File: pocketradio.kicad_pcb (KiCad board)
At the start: 2 copper layers, 30 x 30 mm, 23 parts, among them CN1 PJ-320D, U1 SI4702-C19-GMR, U2 CH32V003F4U6, U3 TPA6130A2RTJR

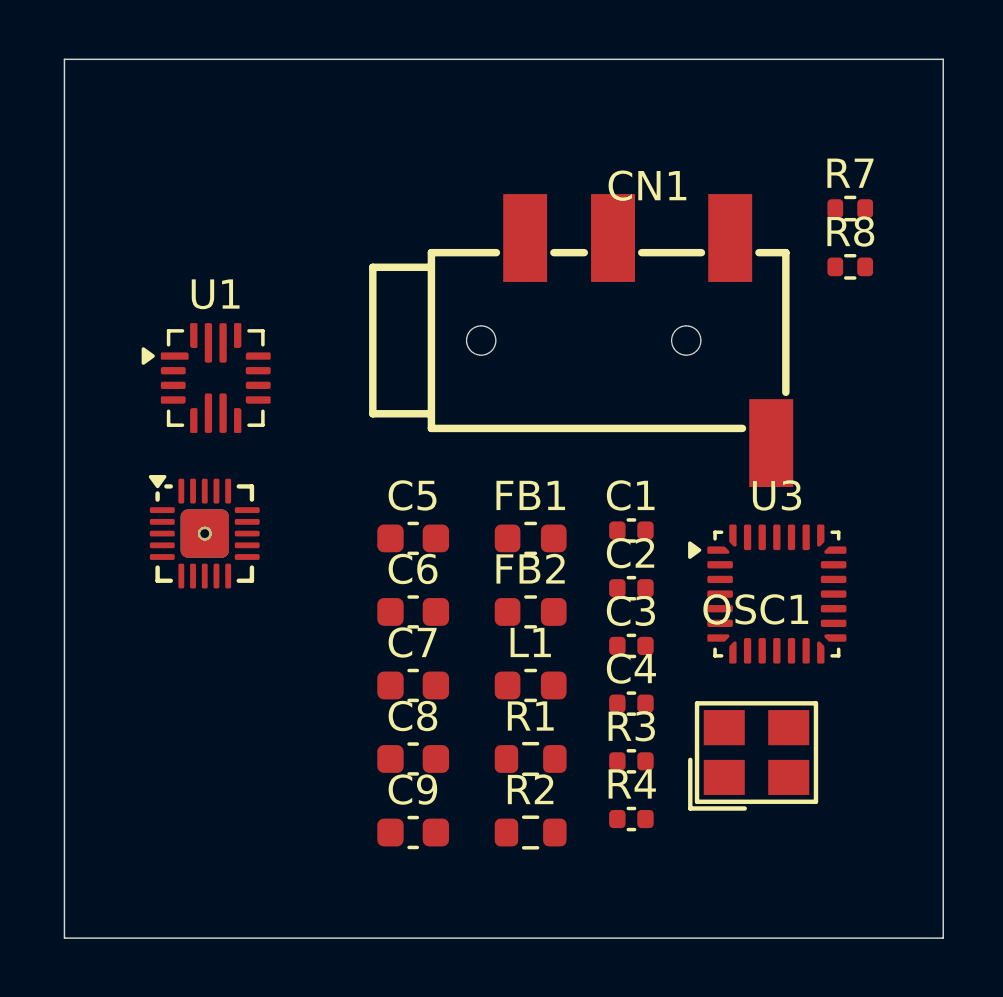
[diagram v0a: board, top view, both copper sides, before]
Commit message: lots of stuff
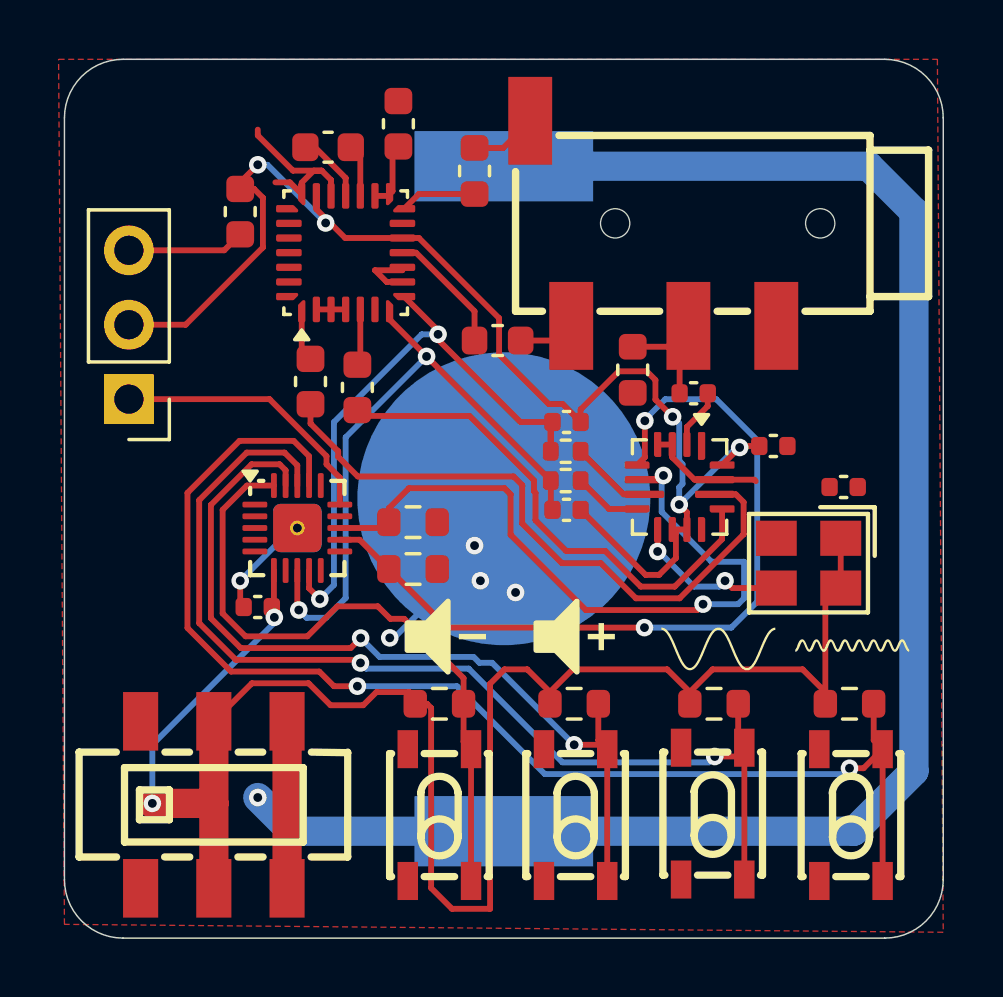
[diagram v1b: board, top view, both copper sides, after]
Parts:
- added BT1: MY-2032-12, easyeda2kicad:BAT-SMD_MY-2032-12, B.Cu at (142.6, 62.2)
- added J1: Conn_01x03_Pin, Connector_PinHeader_2.54mm:PinHeader_1x03_P2.54mm_Vertical, F.Cu at (129.8, 58.8)
- added R1: 10k, Resistor_SMD:R_0603_1608Metric, F.Cu at (149.8, 69.2)
- added R2: 10k, Resistor_SMD:R_0603_1608Metric, F.Cu at (154.4, 69.2)
- added R3: 10k, Resistor_SMD:R_0603_1608Metric, F.Cu at (145.0, 69.2)
- added R4: 10k, Resistor_SMD:R_0603_1608Metric, F.Cu at (140.4, 69.2)
- added SW1: SW_Push_45deg, easyeda2kicad:SW-SMD_4P-L4.2-W3.3-P2.15-LS5.1, F.Cu at (149.7, 73.0)
- added SW2: SW_Push_45deg, easyeda2kicad:SW-SMD_4P-L4.2-W3.3-P2.15-LS5.1, F.Cu at (154.4, 73.0)
- added SW3: SW_Push_45deg, easyeda2kicad:SW-SMD_4P-L4.2-W3.3-P2.15-LS5.1, F.Cu at (145.0, 73.0)
- added SW4: SW_Push_45deg, easyeda2kicad:SW-SMD_4P-L4.2-W3.3-P2.15-LS5.1, F.Cu at (140.4, 73.0)
- added SW5: K3-2235S-F1, easyeda2kicad:SW-SMD_MST22D18G2, F.Cu at (132.7, 72.7)
- moved C7 24.2 mm to (139.0, 49.4), turned to 90 degrees
- moved C8 21.1 mm to (136.6, 50.2)
- moved U2 18.8 mm to (137.2, 53.8), turned to 90 degrees
- moved C5 17.2 mm to (133.6, 52.4), turned to -90 degrees
- moved U3 16.3 mm to (148.6, 61.8), turned to -90 degrees
- moved R8 13.7 mm to (144.7, 59.6), turned to 180 degrees
- moved C1 13.0 mm to (134.2, 65.9), turned to 180 degrees
- moved R9 12.8 mm to (144.7, 60.6)
- moved FB1 12.7 mm to (141.6, 51.0), turned to -90 degrees
- moved R10 12.1 mm to (144.7, 61.6)
- moved R6 11.3 mm to (139.5, 63.0)
- moved L1 11.3 mm to (147.0, 57.8), turned to -90 degrees
- moved C2 10.8 mm to (149.1, 58.6)
- moved FB2 9.33 mm to (142.4, 56.8), turned to 180 degrees
- moved C6 9.05 mm to (154.2, 61.8), turned to 180 degrees
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- renumbered C4 to C2, C5 to C3, C6 to C4, C7 to C5, C3 to C6, C9 to C7, C2 to C9, R8 to R10, R1 to R5, R2 to R6, R3 to R7, R4 to R8, R7 to R9, U2 to U1, U3 to U2, U1 to U3
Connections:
- U1 pad 17: unconnected-(U2-PD3-Pad17) -> /PD3
- U1 pad 18: unconnected-(U2-PD4-Pad18) -> /PD4
- U1 pad 19: unconnected-(U2-PD5-Pad19) -> /PD5
- U1 pad 20: unconnected-(U2-PD6-Pad20) -> /PD6
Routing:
- net +3V3: track 0.00 -> 108.0 mm, vias 0 -> 7
- net Net-(BT1-Pad1): track 0.00 -> 63.2 mm, vias 0 -> 1
- net /PD3: track 0.00 -> 43.0 mm, vias 0 -> 2
- net /PD4: track 0.00 -> 36.0 mm, vias 0 -> 2
- net /PD5: track 0.00 -> 29.4 mm, vias 0 -> 2
- net /RF_RST: track 0.00 -> 27.7 mm, vias 0 -> 2
- net GND: track 0.00 -> 27.6 mm, vias 0 -> 5
- net /SEN: track 0.00 -> 24.1 mm, vias 0 -> 2
- net /PD6: track 0.00 -> 22.6 mm
- net /L_RAW: track 0.00 -> 21.9 mm
- net /SDA: track 0.00 -> 21.9 mm, vias 0 -> 2
- net /SCL: track 0.00 -> 21.4 mm, vias 0 -> 2
- net /R_RAW: track 0.00 -> 17.4 mm
- net /SWDEBUG: track 0.00 -> 9.39 mm
- net /RCLK: track 0.00 -> 5.48 mm, vias 0 -> 2
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- added copper zone on F.Cu, net GND
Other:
- outline, holes or cut-outs redrawn
- board text added: "Designed by Alex Park"
- board text added: "Sussy Radio Keychain Rev 1"
